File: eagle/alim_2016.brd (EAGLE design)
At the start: 66.5 x 50 mm, 74 parts, among them J1 AVR_SPI_PRG_6PTH, U1 3.3V, U4 LM2596S-ADJ, U6 ATMEGA328P_TQFP

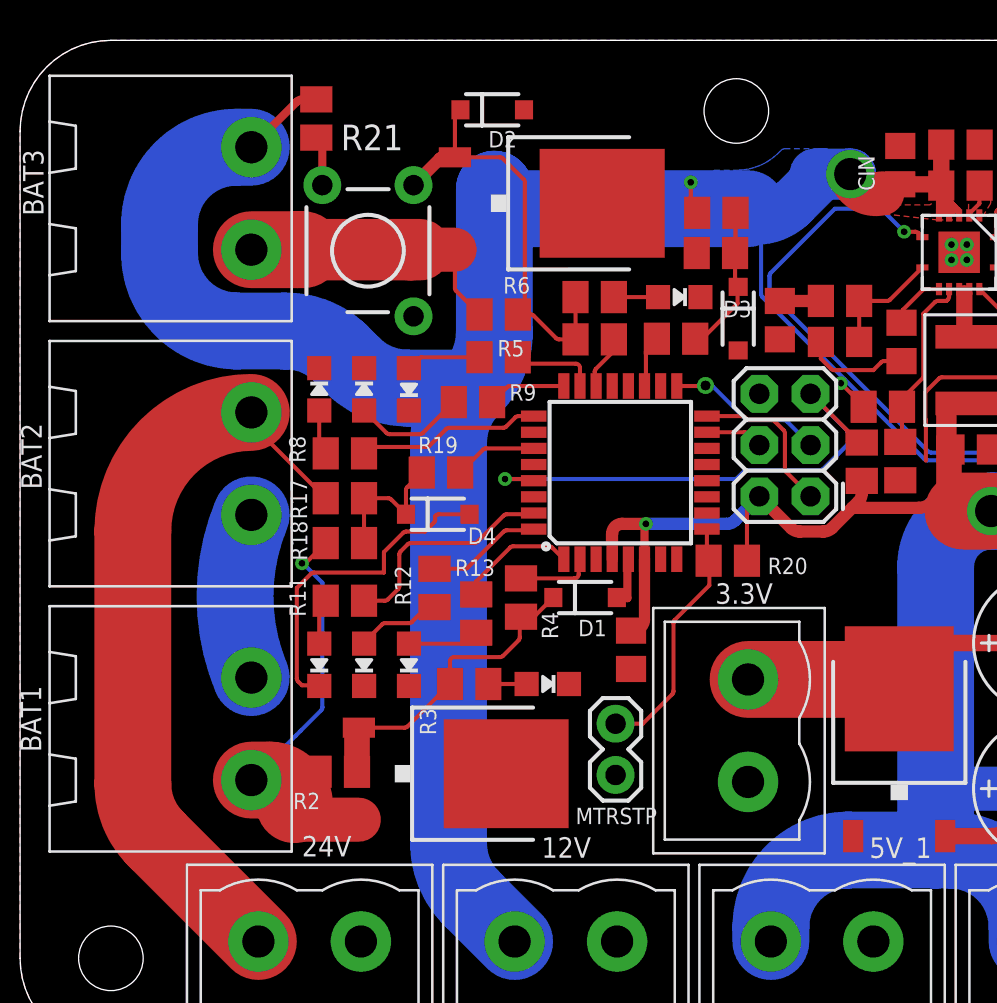
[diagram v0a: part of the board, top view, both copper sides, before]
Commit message: shuffle things around
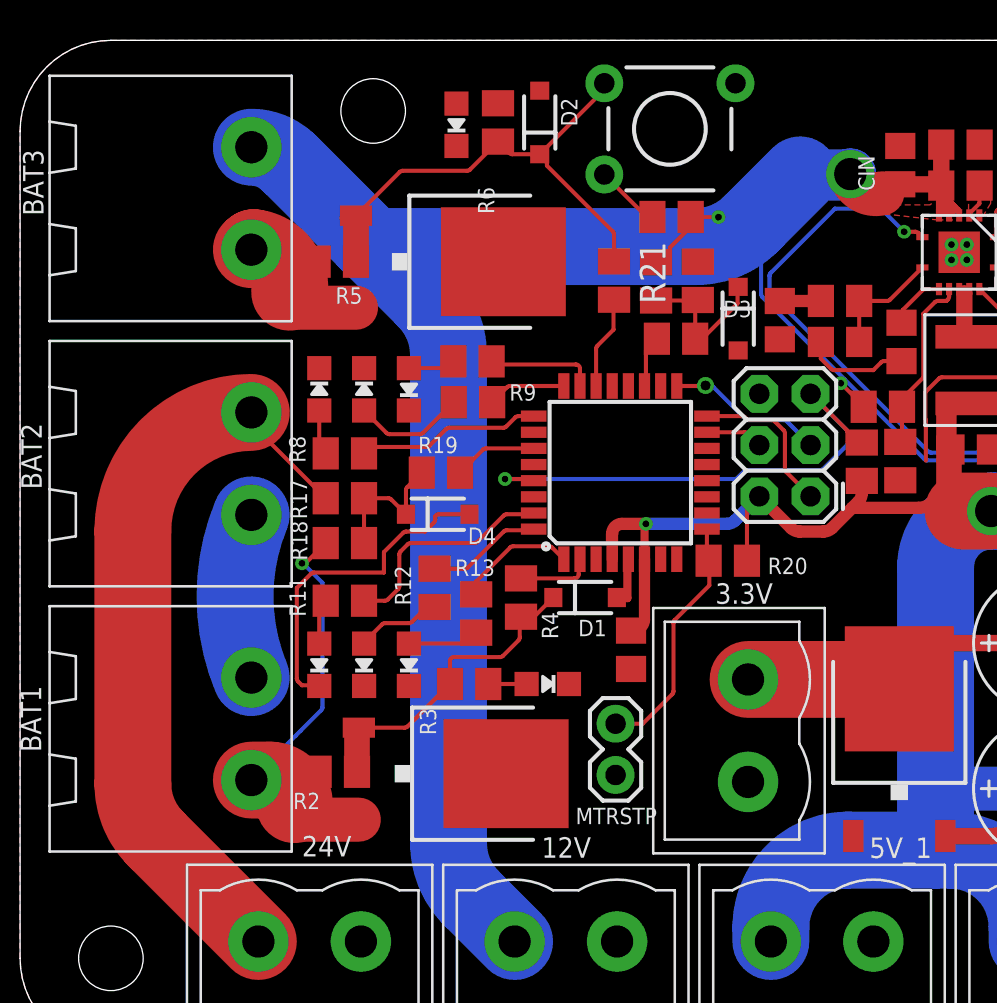
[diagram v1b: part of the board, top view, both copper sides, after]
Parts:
- moved R21 18.3 mm to (32.3, 41.2), turned to 180 degrees
- moved S1 16.1 mm to (32.2, 45.6), turned to 0 degrees
- moved LED7 14.0 mm to (21.6, 45.8), turned to 180 degrees
- moved R6 9.89 mm to (23.7, 45.9), turned to 270 degrees
- moved R5 8.44 mm to (15.7, 39.0)
- moved U$38 5.69 mm to (21.5, 39.0)
- moved R14 4.53 mm to (31.5, 38.1), turned to 90 degrees
- moved R7 3.07 mm to (29.4, 38.1), turned to 270 degrees
- moved D2 2.44 mm to (25.8, 45.9), turned to 90 degrees
- moved R15 1.64 mm to (33.6, 38.1), turned to 270 degrees
- moved R10 1.31 mm to (22.4, 34.1)
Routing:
- net 12V: track 142.4 -> 123.4 mm
- net N$13: track 16.4 -> 10.1 mm
- net BAT12_CUT: track 21.5 -> 25.3 mm
- net N$10: track 2.19 -> 0.00 mm
- net N$23: track 2.71 -> 4.63 mm
- net N$17: track 3.70 -> 2.41 mm
- net N$22: track 4.20 -> 5.39 mm
- net N$7: track 2.48 -> 3.25 mm
- net BAT12_SENSE: track 7.57 -> 8.10 mm
- removed copper zone on layer 16, net 12V
